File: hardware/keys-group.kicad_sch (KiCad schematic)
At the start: 17 parts

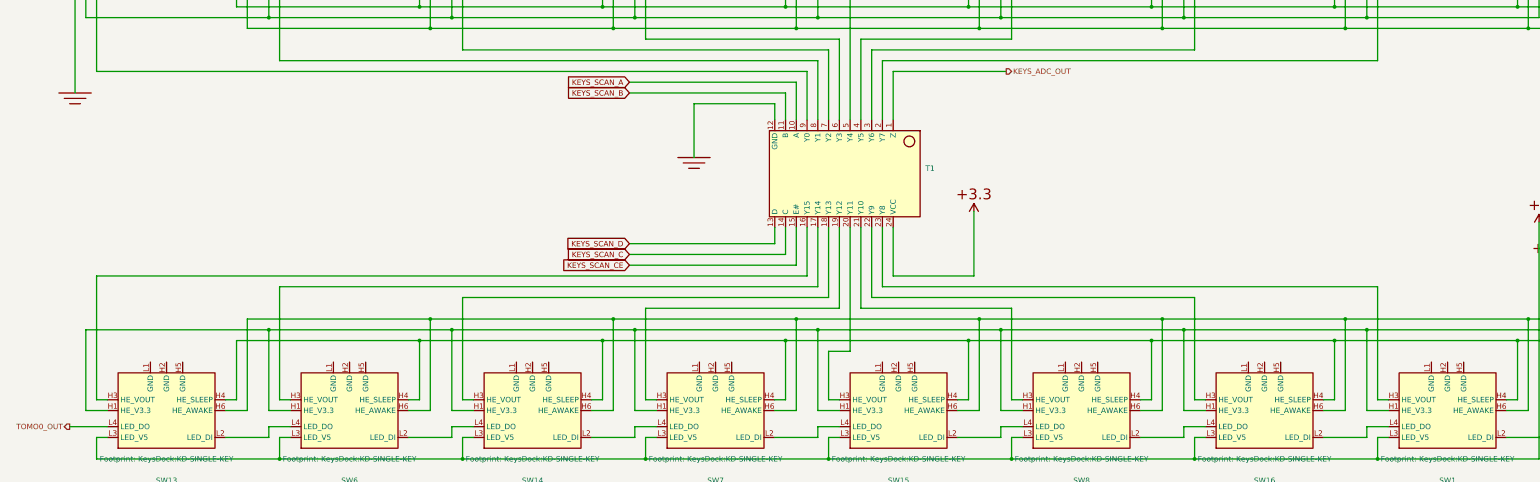
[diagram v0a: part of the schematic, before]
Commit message: :construction: typeboard routing
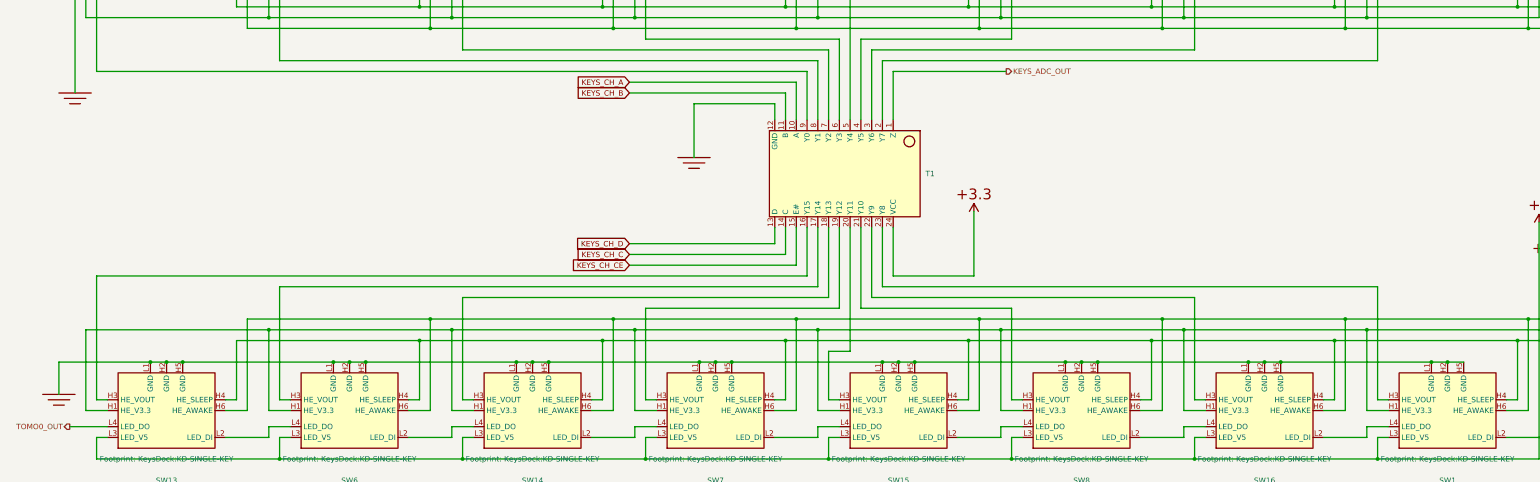
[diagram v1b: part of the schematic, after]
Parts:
- T1: footprint KeysDock:XL4067 -> KeysDock:XL4067TS; symbol components:XL4067 -> components:XL4067TS
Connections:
- net P,E: now also SW1.H2 (GND), SW1.H5 (GND), SW1.L1 (GND), SW13.H2 (GND), SW13.H5 (GND), SW13.L1 (GND), SW14.H2 (GND), SW14.H5 (GND), SW14.L1 (GND), SW15.H2 (GND), SW15.H5 (GND), SW15.L1 (GND), SW16.H2 (GND), SW16.H5 (GND), SW16.L1 (GND), SW6.H2 (GND), SW6.H5 (GND), SW6.L1 (GND), SW7.H2 (GND), SW7.H5 (GND), SW7.L1 (GND), SW8.H2 (GND), SW8.H5 (GND), SW8.L1 (GND)
- net KEYS_SCAN_A renamed KEYS_CH_A
- net KEYS_SCAN_B renamed KEYS_CH_B
- net KEYS_SCAN_C renamed KEYS_CH_C
- net KEYS_SCAN_CE renamed KEYS_CH_CE
- net KEYS_SCAN_D renamed KEYS_CH_D

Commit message: :sparkles: finish 2-piece pcb design
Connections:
- net P,E: no longer SW1.L1 (GND), SW10.L1 (GND), SW11.L1 (GND), SW12.L1 (GND), SW13.L1 (GND), SW14.L1 (GND), SW15.L1 (GND), SW16.L1 (GND), SW2.L1 (GND), SW3.L1 (GND), SW4.L1 (GND), SW5.L1 (GND), SW6.L1 (GND), SW7.L1 (GND), SW8.L1 (GND), SW9.L1 (GND)
- removed net LED_DATA_INNER: SW1.L2 (LED_DI), SW9.L4 (LED_DO)
- removed net P,+5: SW1.L3 (LED_V5), SW10.L3 (LED_V5), SW11.L3 (LED_V5), SW12.L3 (LED_V5), SW13.L3 (LED_V5), SW14.L3 (LED_V5), SW15.L3 (LED_V5), SW16.L3 (LED_V5), SW2.L3 (LED_V5), SW3.L3 (LED_V5), SW4.L3 (LED_V5), SW5.L3 (LED_V5), SW6.L3 (LED_V5), SW7.L3 (LED_V5), SW8.L3 (LED_V5), SW9.L3 (LED_V5)
- removed net TOMO0_IN: SW5.L2 (LED_DI)
- removed net TOMO0_OUT: SW13.L4 (LED_DO)
